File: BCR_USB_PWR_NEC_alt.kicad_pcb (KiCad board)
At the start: 2 copper layers, 32.2 x 17 mm, 2 parts, among them CN1 DB9_Female, CN2 UE27AC54100

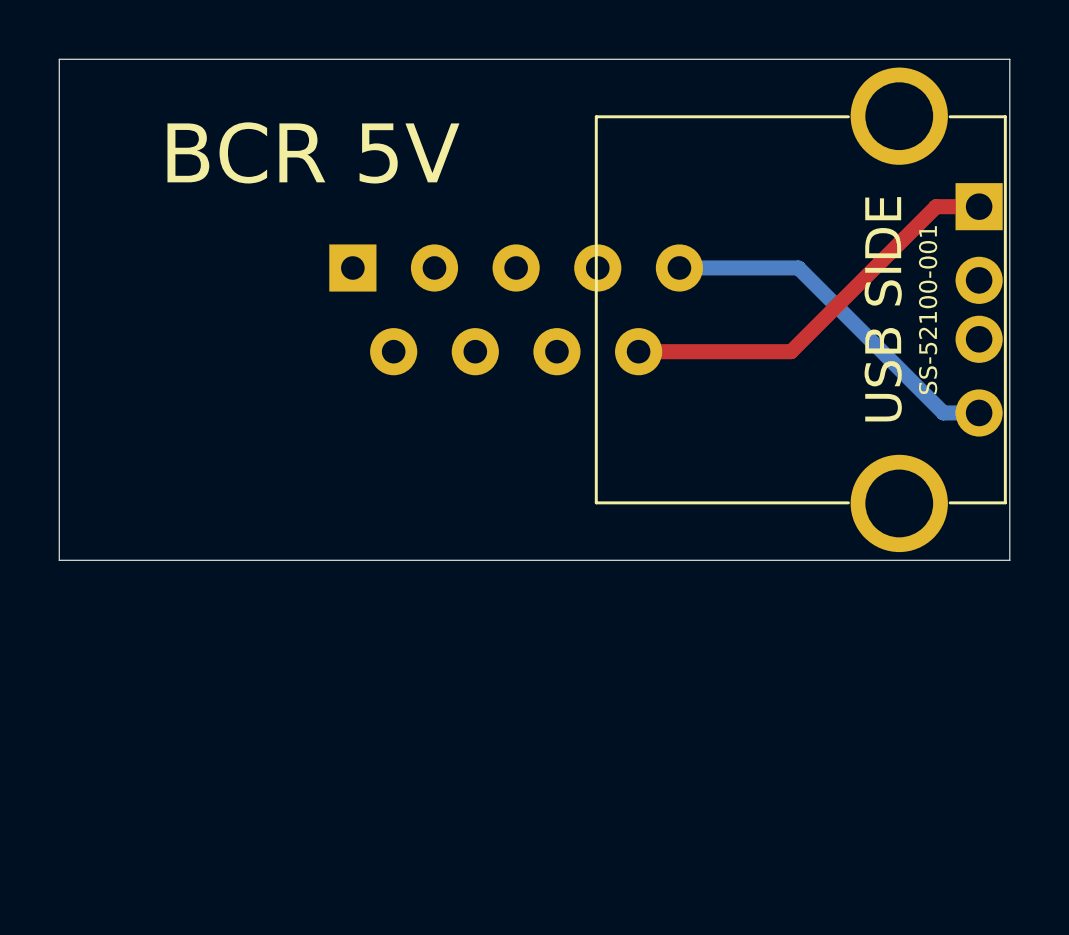
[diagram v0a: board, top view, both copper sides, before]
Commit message: clean up junk files
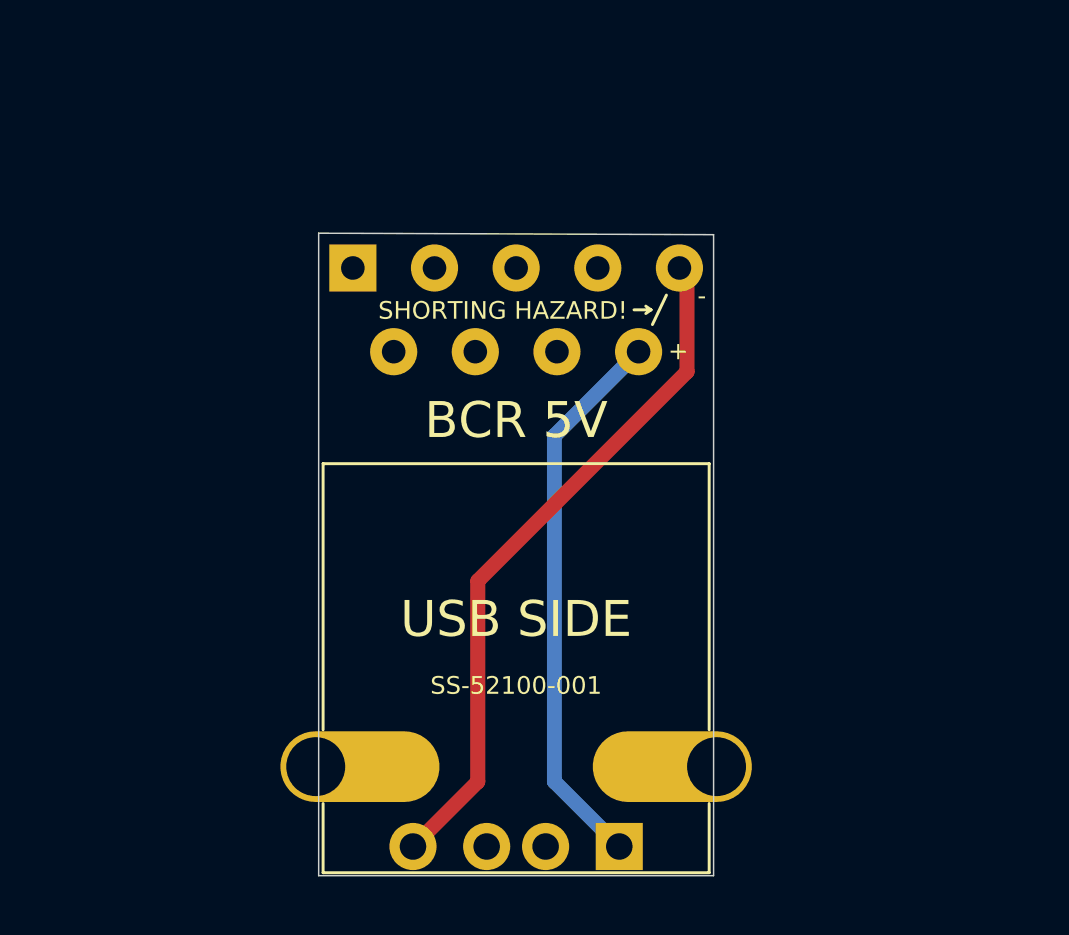
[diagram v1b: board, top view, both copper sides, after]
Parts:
- CN1: footprint 0_LOCAL:TE-5207826 -> 0_LOCAL:TE-5207826_nec
- CN2: footprint 0_LOCAL:USB_A_Female_UE27AC54100 -> 0_LOCAL:USB_A_Female_UE27AC54100_cut
- moved CN2 20.2 mm to (127.0, 111.3), turned to 180 degrees
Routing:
- net /GND: track 12.2 -> 23.6 mm
- net /+5V: track 13.6 -> 18.9 mm
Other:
- board size 32.2 x 17 mm -> 13.4 x 21.8 mm
- board text added: "+"
- board text added: "-"
- board text added: "5v USB power"
- board text added: "NEC PC-8201 / PC-8300"
- board text added: "SHORTING HAZARD!"
- board text added: "from BCR port"
- board text removed: "5v USB power from BCR port"
- board text removed: "TRS-80 Model 100 / TANDY 200"
